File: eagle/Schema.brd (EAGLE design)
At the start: 51.7 x 57.1 mm, 31 parts, among them IC1 TL072P, IC2 MEGA8-P, J1 POWER_JACKSLT, Q1 16MHz

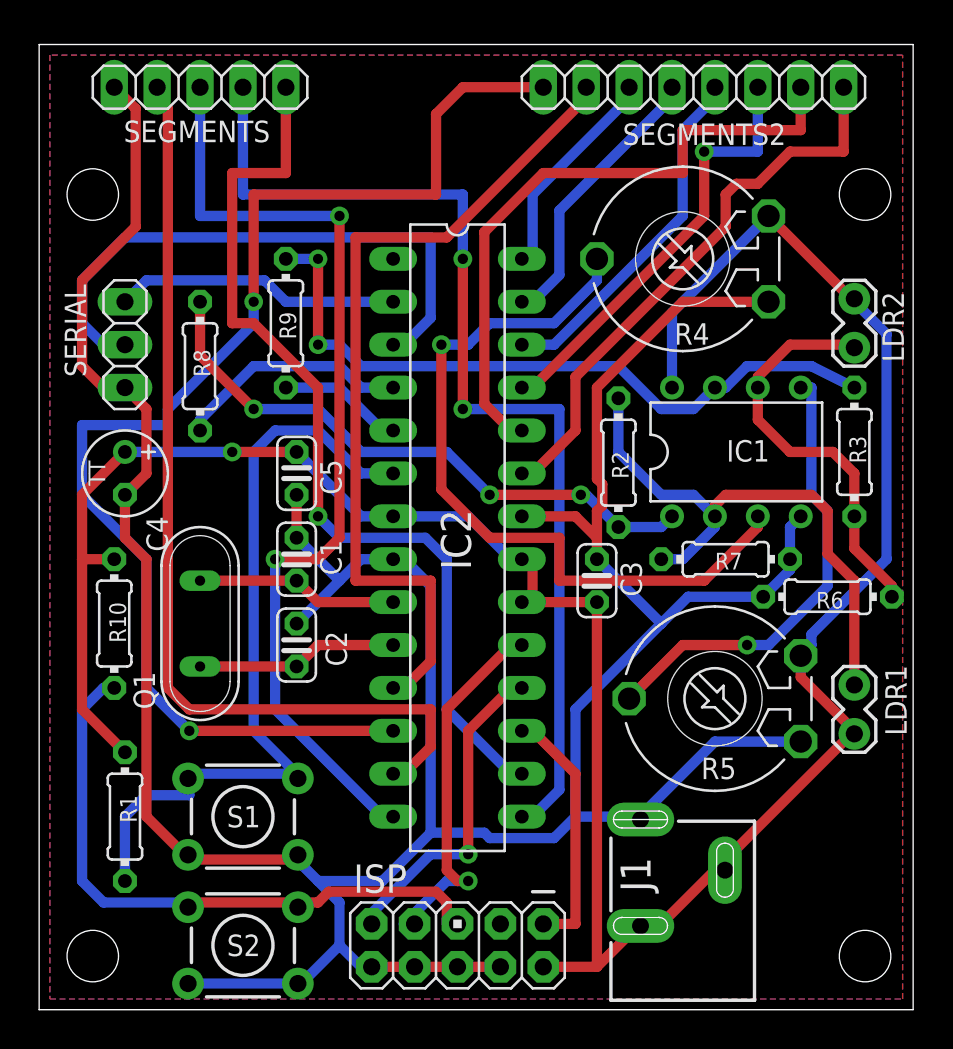
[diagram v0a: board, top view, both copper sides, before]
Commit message: Updated schematics
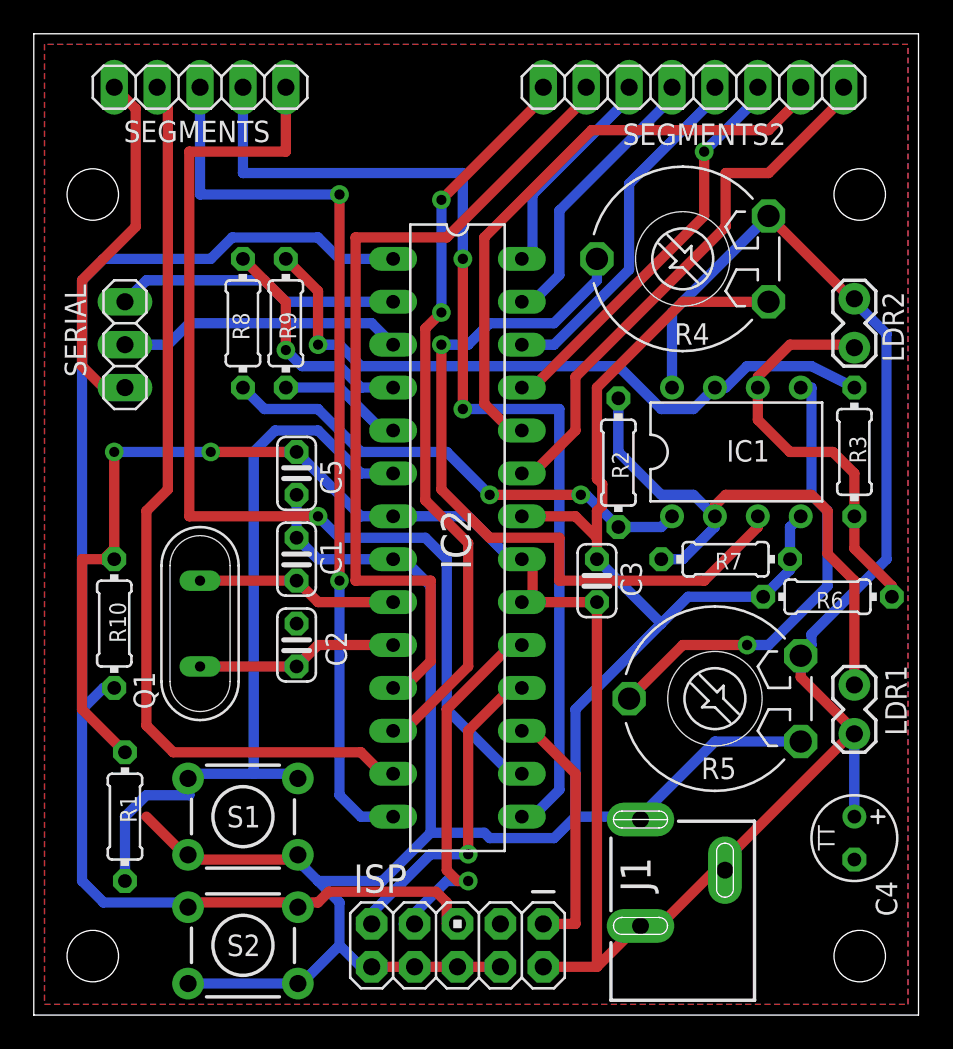
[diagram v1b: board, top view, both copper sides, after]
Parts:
- moved C4 48.3 mm to (47.0, 10.2)
- moved R8 3.59 mm to (10.8, 40.6), turned to 270 degrees
- moved U$4 0.32 mm to (47.3, 48.3)
- moved U$5 0.32 mm to (47.3, 3.17)
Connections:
- net RESET: now also IC2.1
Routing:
- net RESET: track 38.0 -> 83.4 mm
- net N$20: track 76.2 -> 44.3 mm
- net GND: track 208.9 -> 177.3 mm
- net N$4: track 34.9 -> 18.8 mm
- net N$11: track 55.0 -> 62.3 mm
- net N$3: track 35.6 -> 29.1 mm, vias 3 -> 2
- net +5V: track 151.9 -> 156.7 mm, vias 1 -> 2
- net N$13: track 57.8 -> 54.5 mm
- net N$15: track 38.3 -> 35.5 mm
- net N$22: track 57.0 -> 55.0 mm
- net N$16: track 25.8 -> 23.9 mm
- net SEGMENTS: track 33.7 -> 32.6 mm
- net N$6: track 41.7 -> 40.5 mm, vias 2 -> 1
- net MODE: track 46.5 -> 45.4 mm
- net PD2: track 13.9 -> 13.7 mm, vias 0 -> 1
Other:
- board size 51.7 x 57.1 mm -> 52.4 x 58.1 mm
